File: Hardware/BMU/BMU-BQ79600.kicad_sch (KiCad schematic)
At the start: 9 parts, among them U4 BQ79600PWRQ1

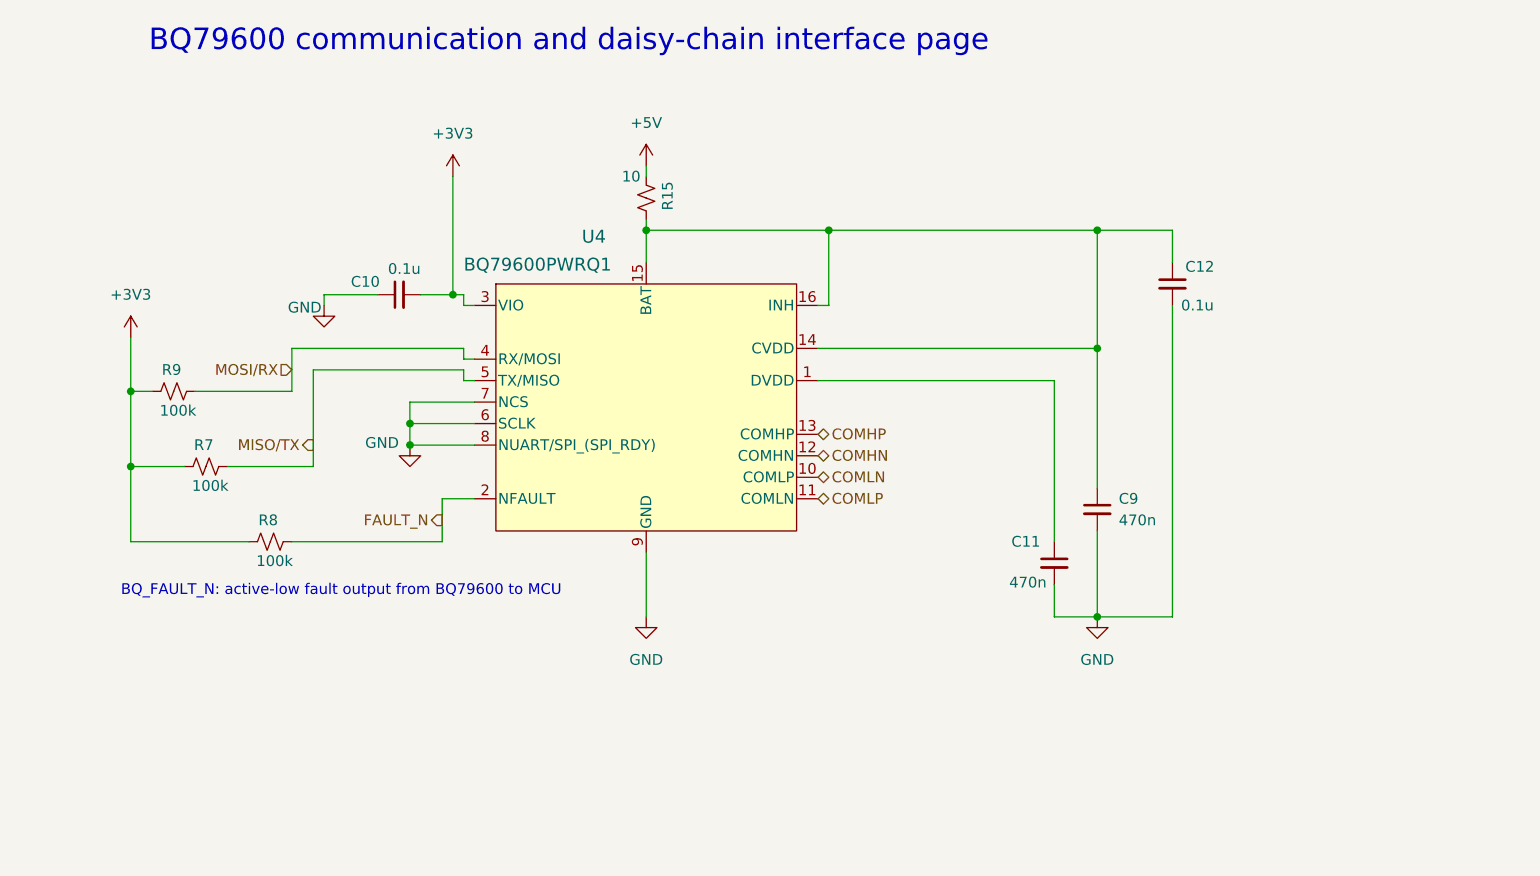
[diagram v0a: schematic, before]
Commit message: add comment
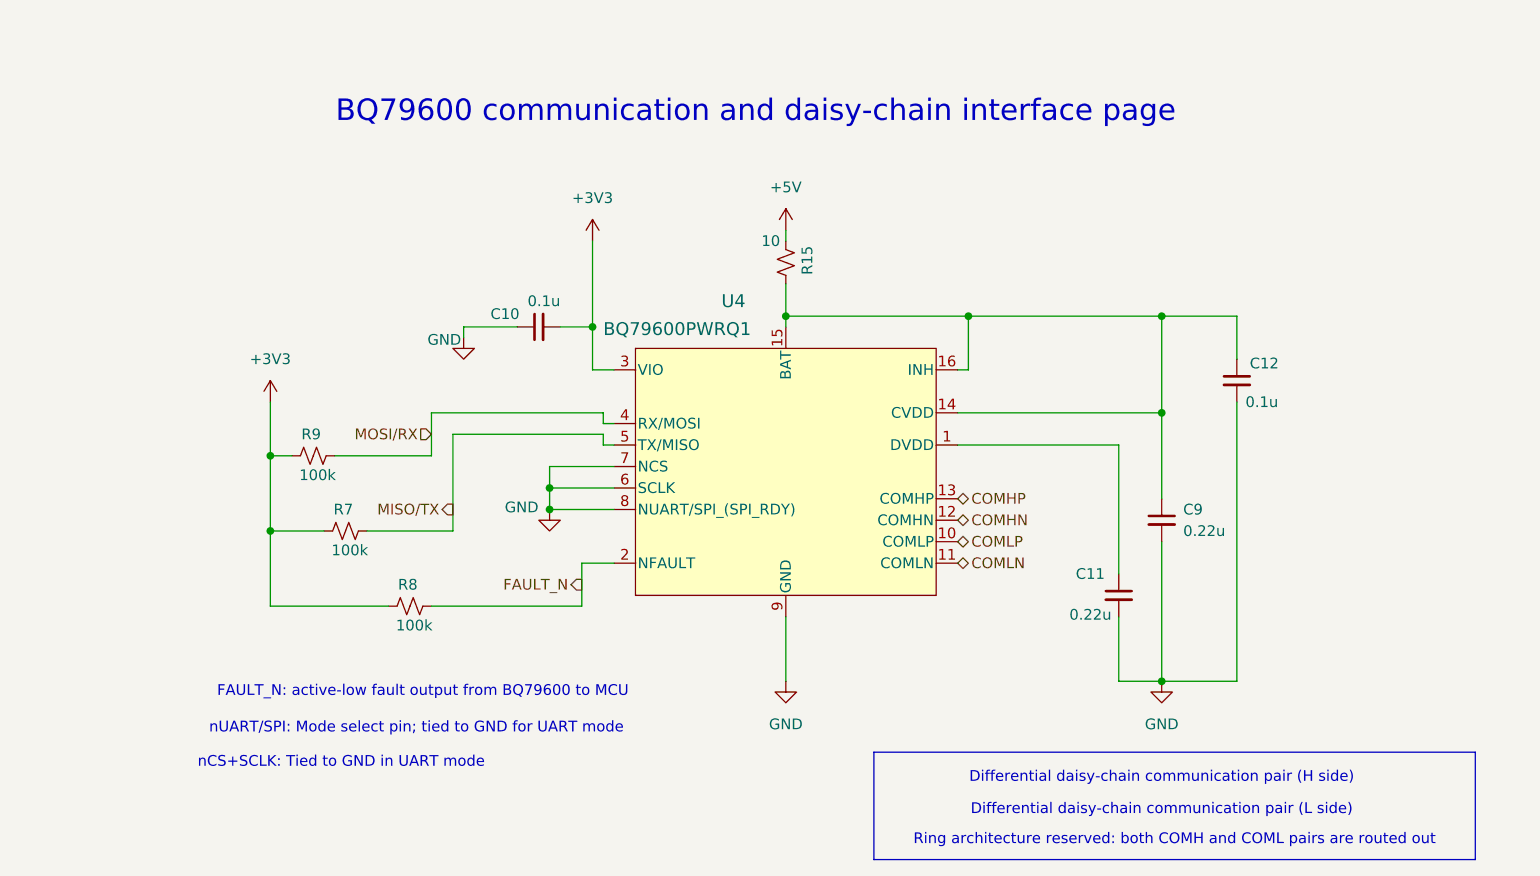
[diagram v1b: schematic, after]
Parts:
- C11, C9: value 470n -> 0.22u
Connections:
- net COMLN: now also U4.11 (COMLN); no longer U4.10 (COMLP)
- net COMLP: now also U4.10 (COMLP); no longer U4.11 (COMLN)
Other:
- note added: "Differential daisy-chain communication pair (H side)"
- note added: "Differential daisy-chain communication pair (L side)"
- note added: "FAULT_N: active-low fault output from BQ79600 to MCU"
- note added: "Ring architecture reserved: both COMH and COML pairs are routed out"
- note added: "nCS+SCLK: Tied to GND in UART mode"
- note added: "nUART/SPI: Mode select pin; tied to GND for UART mode"
- note removed: "BQ_FAULT_N: active-low fault output from BQ79600 to MCU"
- moved on the sheet: C10, C11, C12, C9, R15, R7, R8, R9, U4

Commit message: add footprint
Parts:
- C10, C11, C12, C9: footprint (none) -> Capacitor_SMD:C_0805_2012Metric
- R15, R7, R8, R9: footprint (none) -> Resistor_SMD:R_0805_2012Metric
- U4: footprint TSSOP16_PW_TEX -> BQ79600:TSSOP16_PW_TEX
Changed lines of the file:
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@@
 			)
 		)
-		(property "Footprint" ""
+		(property "Footprint" "Resistor_SMD:R_0805_2012Metric"
 			(at 201.93 118.11 0)
 			(hide yes)
@@
 			)
 		)
-		(property "Footprint" ""
+		(property "Footprint" "Resistor_SMD:R_0805_2012Metric"
 			(at 146.05 140.97 0)
 			(hide yes)
@@
 			)
 		)
-		(property "Footprint" ""
+		(property "Footprint" "Capacitor_SMD:C_0805_2012Metric"
 			(at 241.3 157.48 0)
 			(hide yes)
@@
 			)
 		)
-		(property "Footprint" ""
+		(property "Footprint" "Capacitor_SMD:C_0805_2012Metric"
 			(at 172.72 125.73 0)
 			(hide yes)
@@
 			)
 		)
-		(property "Footprint" "TSSOP16_PW_TEX"
+		(property "Footprint" "BQ79600:TSSOP16_PW_TEX"
 			(at 173.99 132.08 0)
 			(hide yes)
@@
 			)
 		)
-		(property "Footprint" ""
+		(property "Footprint" "Resistor_SMD:R_0805_2012Metric"
 			(at 149.86 149.86 0)
 			(hide yes)
@@
 			)
 		)
-		(property "Footprint" ""
+		(property "Footprint" "Capacitor_SMD:C_0805_2012Metric"
 			(at 255.27 132.08 0)
 			(hide yes)
@@
 			)
 		)
-		(property "Footprint" ""
+		(property "Footprint" "Resistor_SMD:R_0805_2012Metric"
 			(at 157.48 158.75 0)
 			(hide yes)
@@
 			)
 		)
-		(property "Footprint" ""
+		(property "Footprint" "Capacitor_SMD:C_0805_2012Metric"
 			(at 246.38 148.59 0)
 			(hide yes)
